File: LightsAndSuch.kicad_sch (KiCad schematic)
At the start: 13 parts, among them U1 STM32F205RBTx, U2 MAX98357A

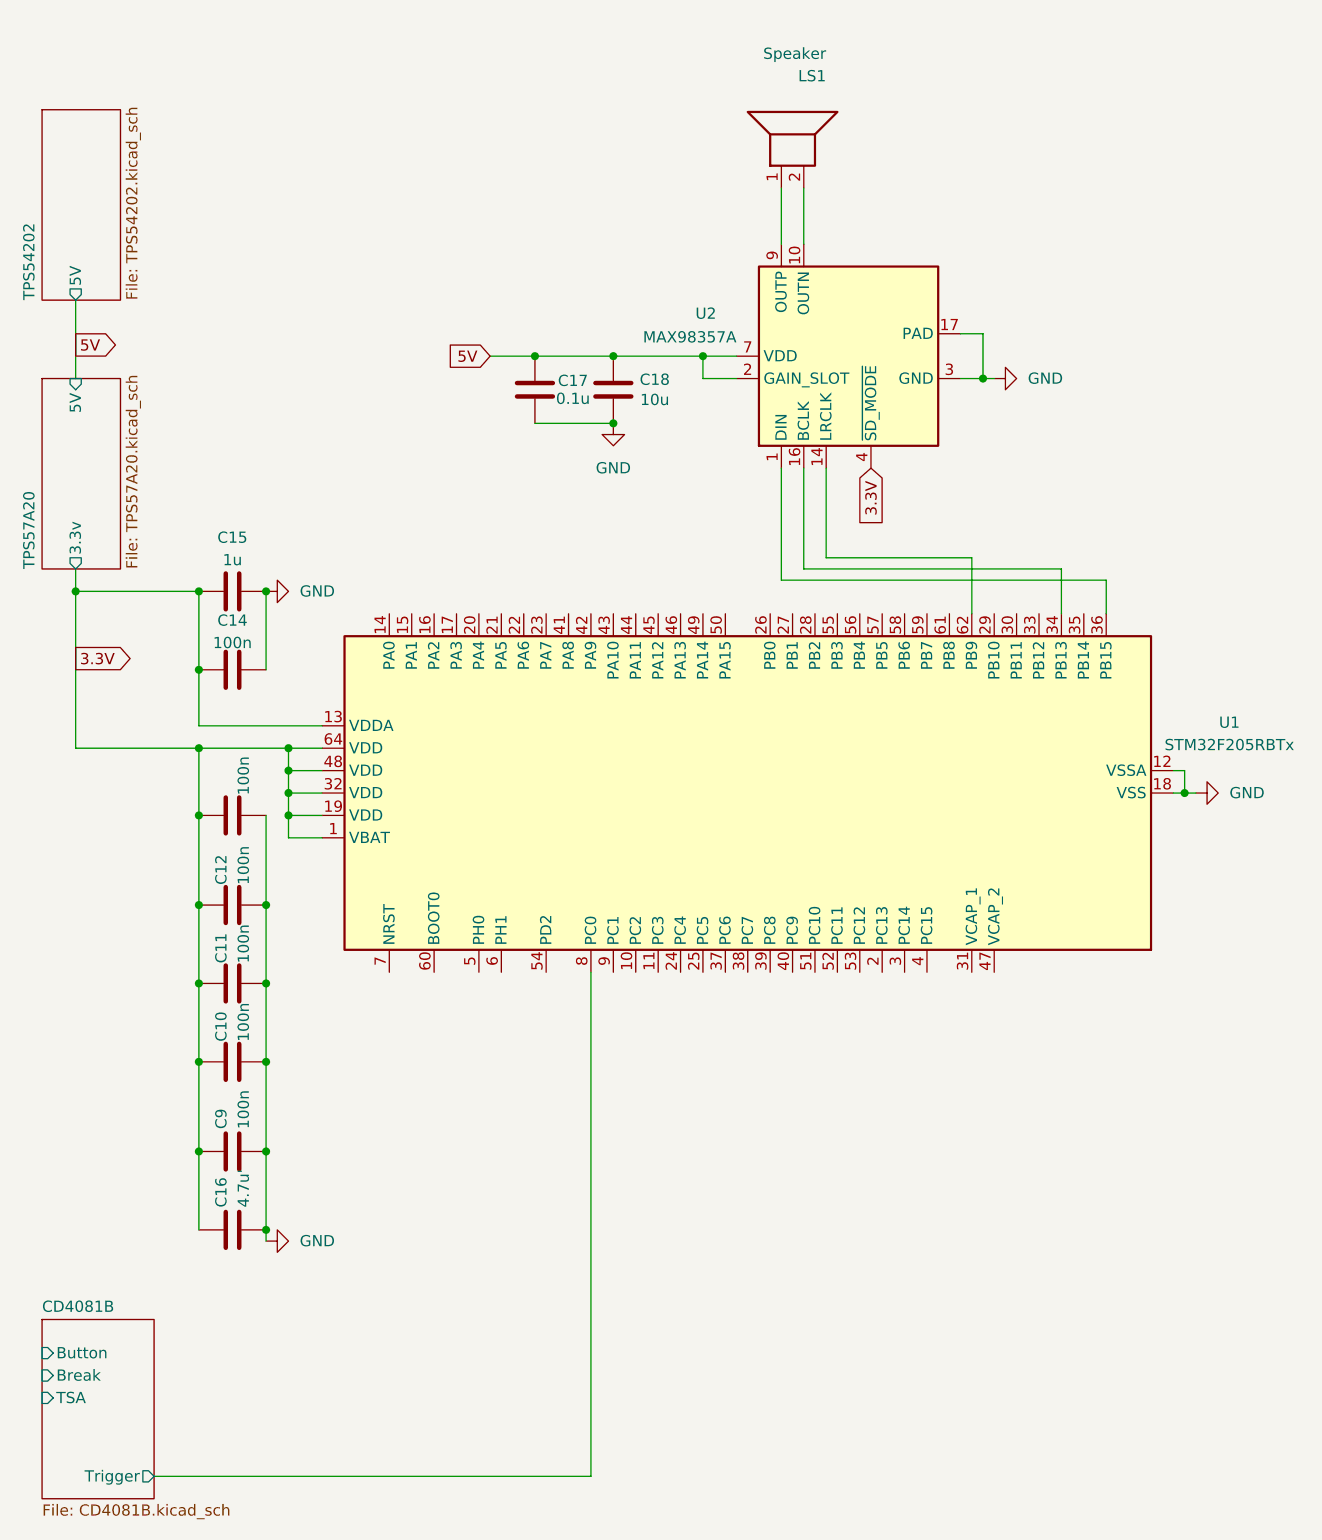
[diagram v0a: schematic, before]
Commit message: added secondary circuit
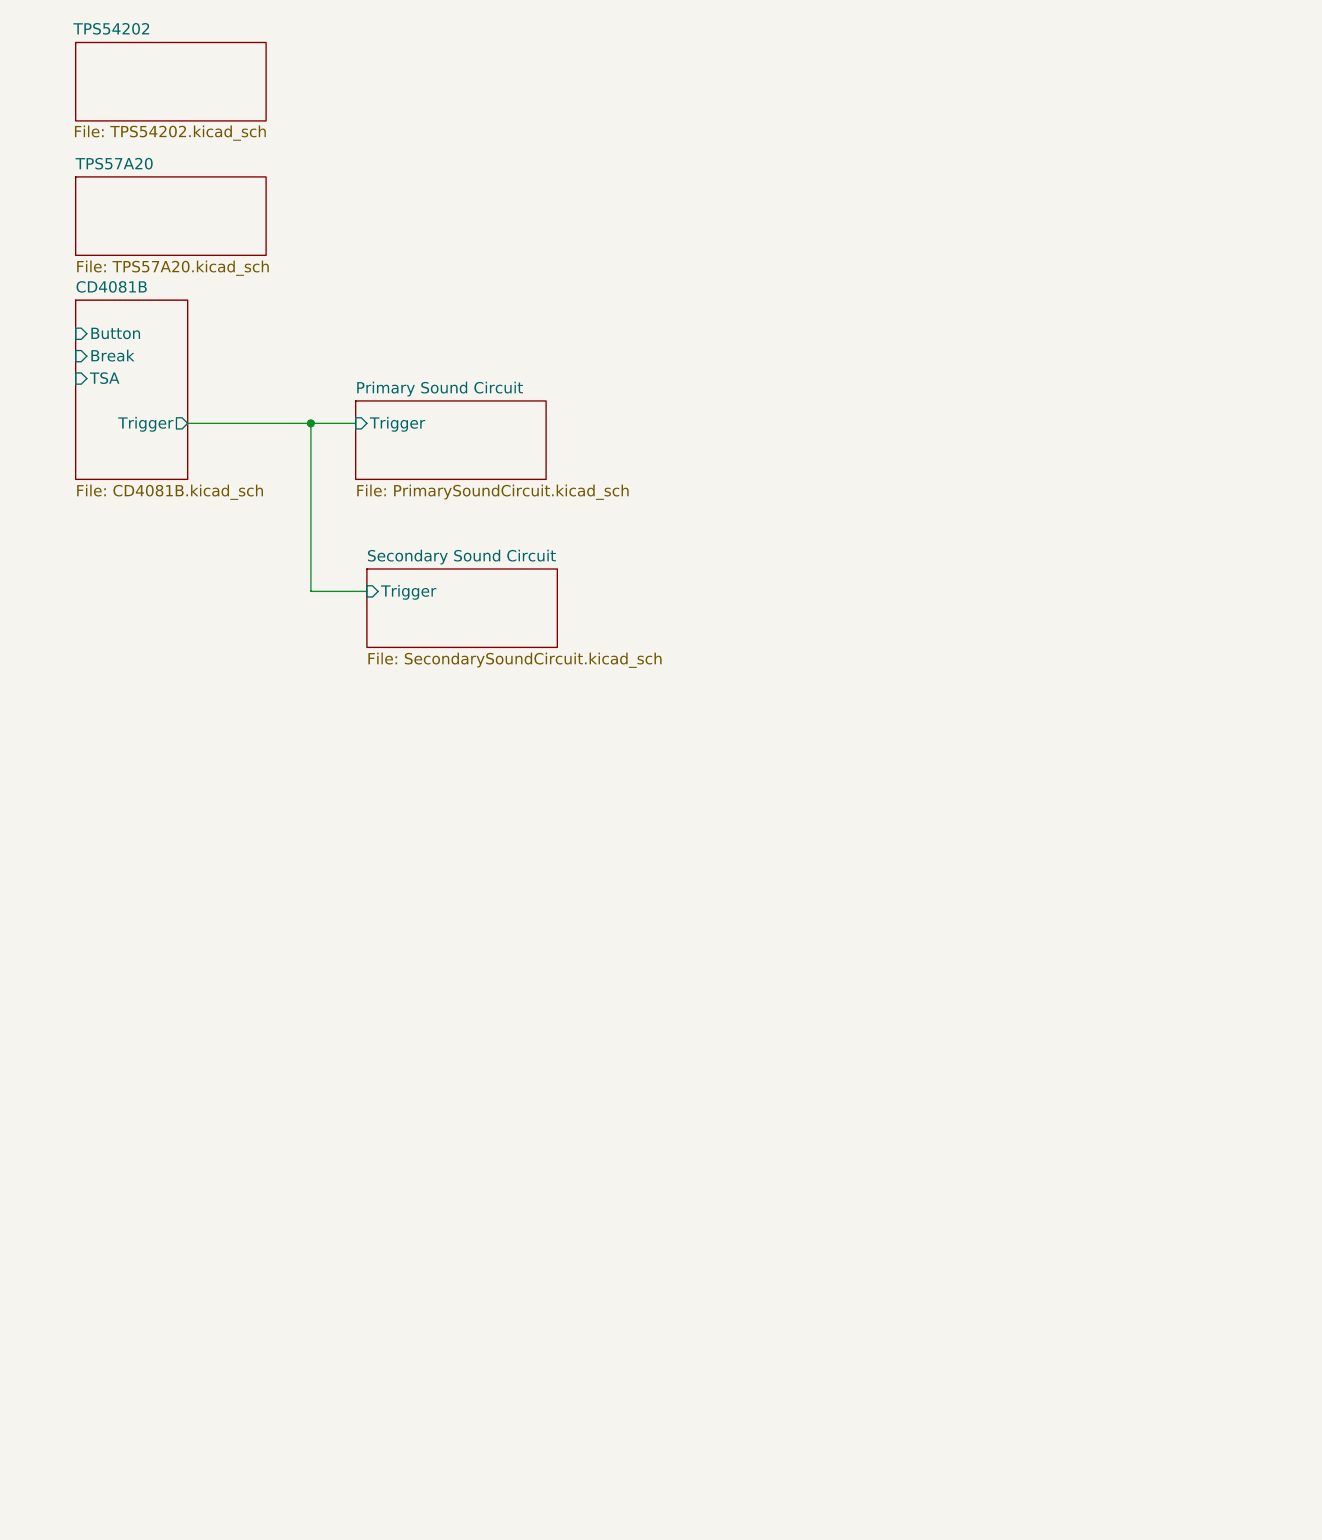
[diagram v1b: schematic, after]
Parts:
- removed C10, C11, C12, C13, C14, C9: 100n, symbol Device:C
- removed C15: 1u, symbol Device:C
- removed C16: 4.7u', symbol Device:C
- removed C17: 0.1u, symbol Device:C
- removed C18: 10u, symbol Device:C
- removed LS1: Speaker, symbol Device:Speaker
- removed U1: STM32F205RBTx, Package_QFP:LQFP-64_10x10mm_P0.5mm, symbol MCU_ST_STM32F2:STM32F205RBTx
- removed U2: MAX98357A, Package_DFN_QFN:TQFN-16-1EP_3x3mm_P0.5mm_EP1.23x1.23mm, symbol Audio:MAX98357A
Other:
- added sheet Primary Sound Circuit (PrimarySoundCircuit.kicad_sch)
- added sheet Secondary Sound Circuit (SecondarySoundCircuit.kicad_sch)
- sheet TPS54202 ports: added none; removed 5V
- sheet TPS57A20 ports: added none; removed 3.3v, 5V
